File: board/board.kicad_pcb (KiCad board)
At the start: 2 copper layers, 13 parts, among them J1 Conn_01x19, J2 Conn_01x19, J3 Conn_01x02, U1 ESP32-WROVER-E, U2 AOZ1280CI

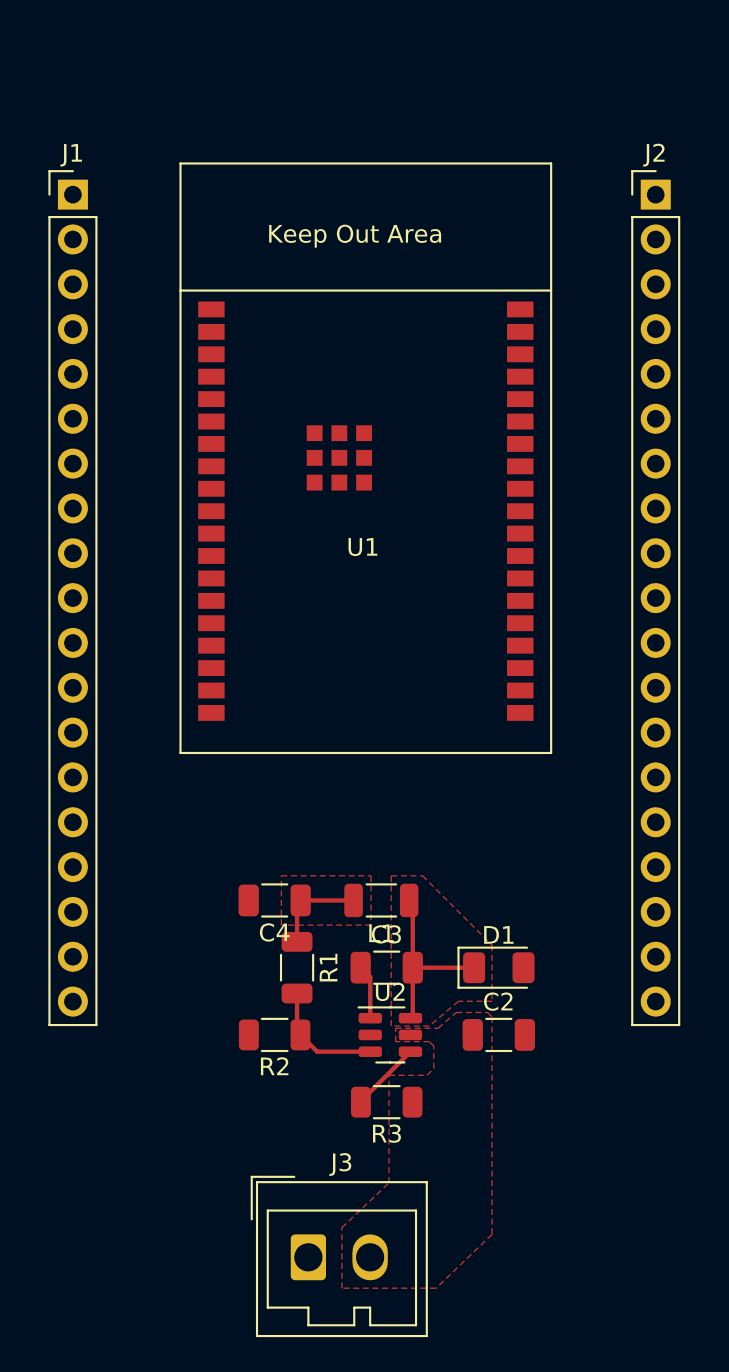
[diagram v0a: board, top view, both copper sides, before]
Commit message: dev
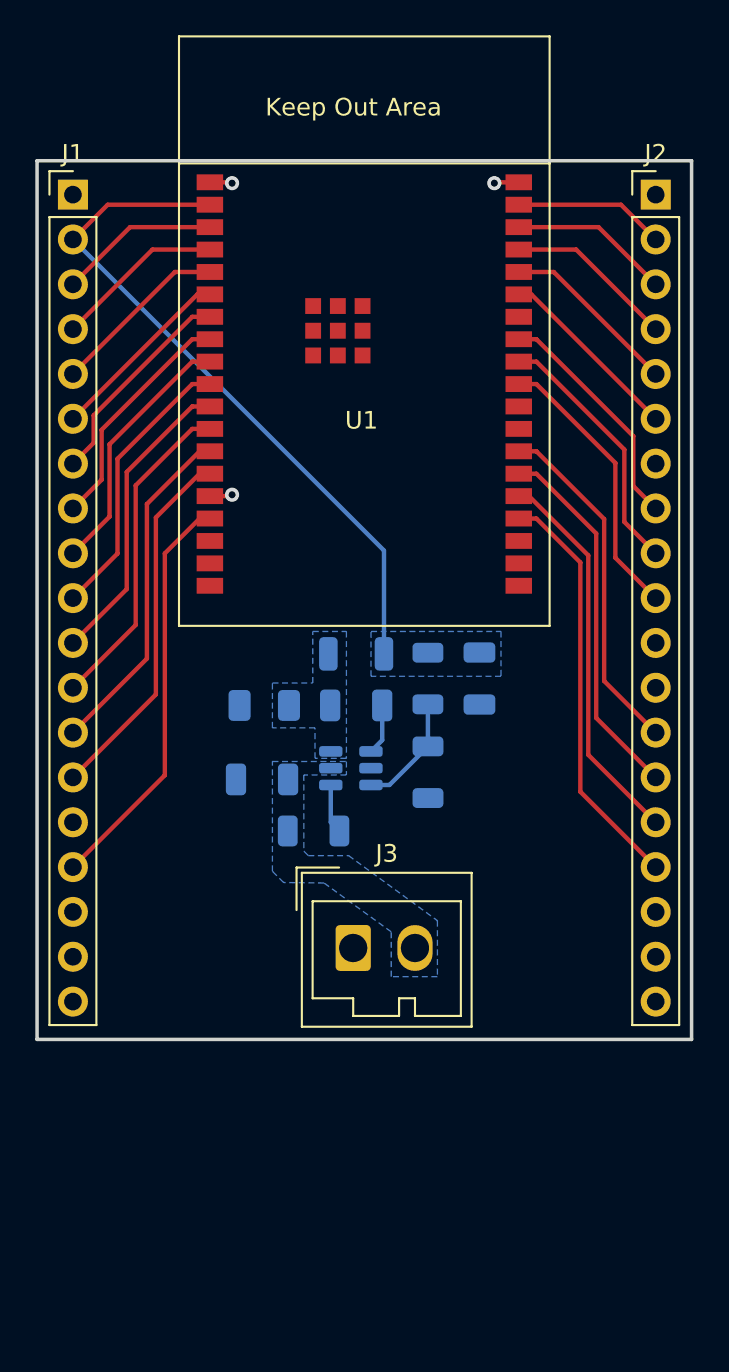
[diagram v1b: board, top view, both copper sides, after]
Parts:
- C2, C3, C4, D1, L1, R1, R2, R3, U2: moved to B.Cu
- moved D1 19.9 mm to (148.0, 84.2), turned to 180 degrees
- moved C2 19.7 mm to (147.9, 88.4), turned to 180 degrees
- moved R1 18.0 mm to (157.3, 82.7)
- moved J3 17.7 mm to (153.0, 97.9)
- moved R2 17.2 mm to (157.3, 88.0), turned to -90 degrees
- moved C4 17.1 mm to (160.2, 82.7), turned to -90 degrees
- moved R3 15.9 mm to (150.8, 91.3), turned to 0 degrees
- moved U2 15.3 mm to (152.9, 87.8), turned to 180 degrees
- moved C3 15.0 mm to (153.2, 84.2), turned to 180 degrees
- moved L1 14.0 mm to (153.2, 81.3), turned to 0 degrees
- moved U1 7.20 mm to (153.7, 66.0)
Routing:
- net 3.3: track 5.43 -> 39.4 mm
- net Net-(J2-Pin_16): track 0.00 -> 23.5 mm
- net Net-(J1-Pin_16): track 0.00 -> 23.3 mm
- net Net-(J2-Pin_15): track 0.00 -> 22.0 mm
- net Net-(J2-Pin_14): track 0.00 -> 21.0 mm
- net Net-(J1-Pin_14): track 0.00 -> 20.8 mm
- net Net-(J2-Pin_13): track 0.00 -> 19.7 mm
- net Net-(J1-Pin_13): track 0.00 -> 19.5 mm
- net Net-(J1-Pin_12): track 0.00 -> 18.5 mm
- net Net-(J1-Pin_11): track 0.00 -> 17.2 mm
- net Net-(J2-Pin_10): track 0.00 -> 15.9 mm
- net Net-(J1-Pin_10): track 0.00 -> 15.9 mm
- net Net-(J2-Pin_9): track 0.00 -> 14.7 mm
- net Net-(J1-Pin_9): track 0.00 -> 14.7 mm
- net Net-(J2-Pin_8): track 0.00 -> 13.4 mm
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- added copper zone on B.Cu, net /VIN
- added copper zone on B.Cu, net /VOUT
- added copper zone on B.Cu, net 3.3
- added copper zone on B.Cu, net GND
- removed copper zone on F.Cu, net /VIN
- removed copper zone on F.Cu, net /VOUT
- removed copper zone on F.Cu, net 3.3
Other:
- board outline added: 37.1 x 49.8 mm

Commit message: dev
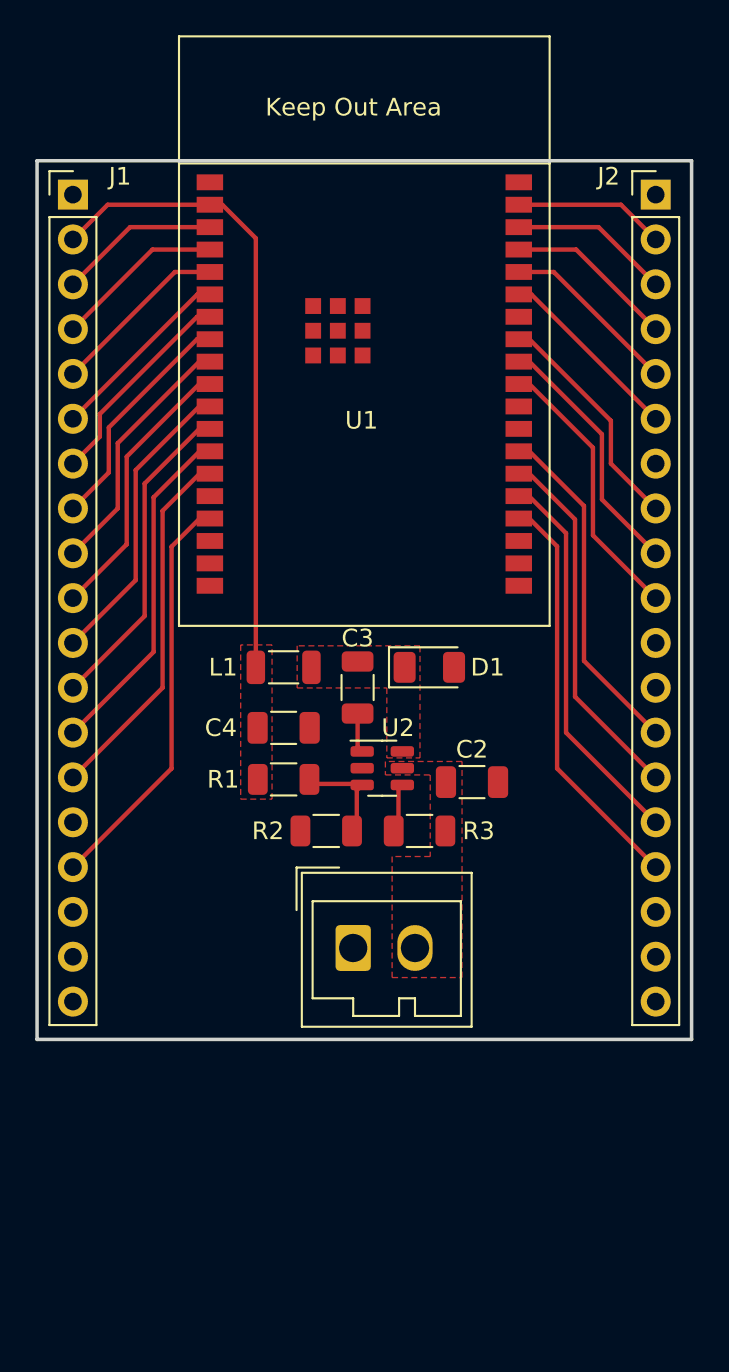
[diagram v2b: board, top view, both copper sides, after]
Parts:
- C2, C3, C4, D1, L1, R1, R2, R3, U2: moved to F.Cu
- moved C2 11.9 mm to (159.8, 88.5), turned to 0 degrees
- moved C4 11.4 mm to (149.1, 85.5), turned to 0 degrees
- moved R1 9.97 mm to (149.1, 88.4), turned to 0 degrees
- moved D1 9.60 mm to (157.4, 82.0), turned to 0 degrees
- moved R2 6.66 mm to (151.5, 91.3), turned to 180 degrees
- moved R3 6.00 mm to (156.8, 91.3), turned to 180 degrees
- moved L1 4.18 mm to (149.1, 82.0), turned to 180 degrees
- moved U2 1.78 mm to (154.7, 87.8), turned to 0 degrees
- moved C3 1.02 mm to (153.3, 83.2), turned to 90 degrees
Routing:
- net GND: track 3.97 -> 0.00 mm, vias 3 -> 0
- net 3.3: track 39.4 -> 36.3 mm
- net Net-(U2-BST): track 2.87 -> 2.25 mm
- net Net-(U2-FB): track 6.52 -> 5.96 mm
- added copper zone on F.Cu, net /VIN
- added copper zone on F.Cu, net /VOUT
- added copper zone on F.Cu, net 3.3
- added copper zone on F.Cu, net GND
- removed copper zone on B.Cu, net /VIN
- removed copper zone on B.Cu, net /VOUT
- removed copper zone on B.Cu, net 3.3

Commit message: dev
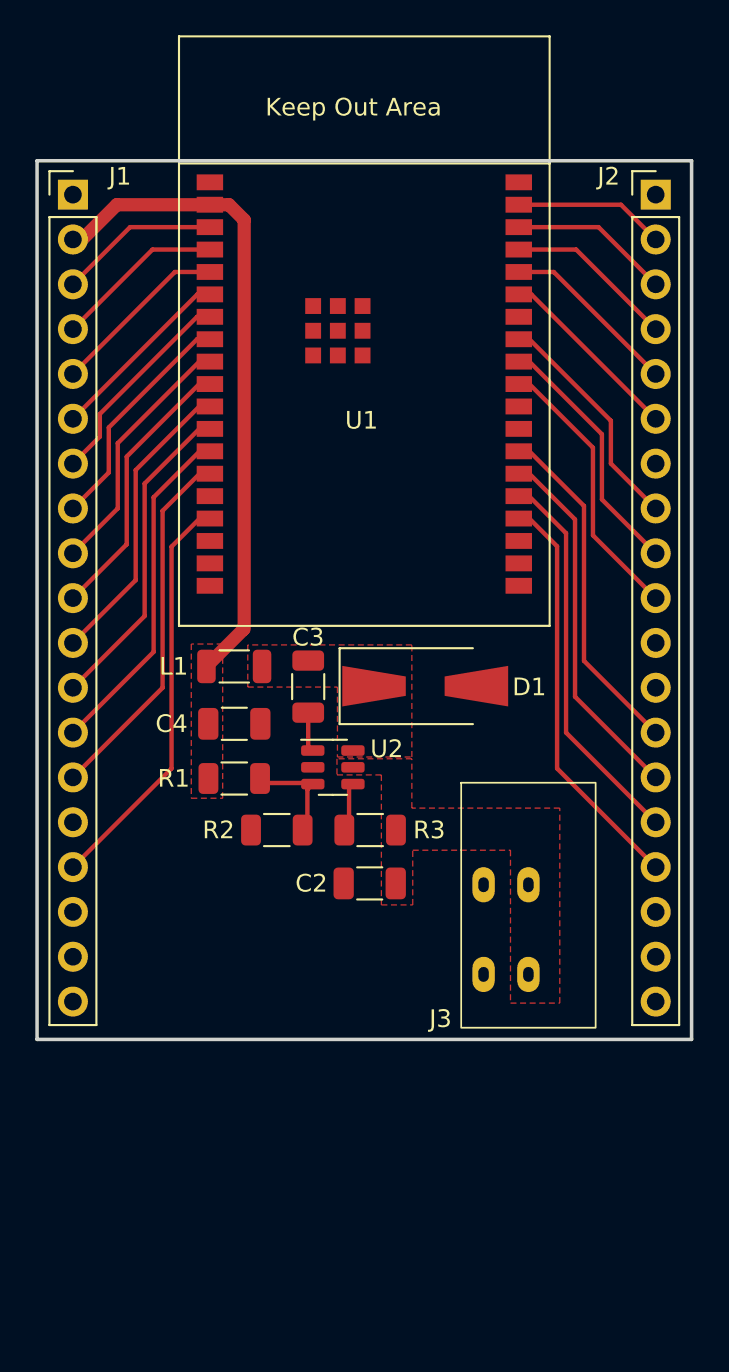
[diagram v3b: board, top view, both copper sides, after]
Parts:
- C2: value C_Small -> 4.7uF
- C3: value C_Small -> 10nF
- C4: value C_Small -> 10uF
- D1: value D_Schottky -> Schottky SMA-SMB; footprint Diode_SMD:D_1206_3216Metric -> Diode_SMD:D_SMA-SMB_Universal_Handsoldering
- J3: value Conn_01x02 -> 3.3-26V; footprint Connector_Wago:Wago_734-132_1x02_P3.50mm_Vertical -> Custom_Connector:Ninigi AC141R-02P-2.54
- L1: value L -> 2.2uH
- R1: value R_Small -> 49.9kΩ
- R2: value R_Small -> 15.8kΩ
- U1: footprint RF_Module_Custom:ESP32-WROVER-IE -> Custom_RF_Module:ESP32-WROVER-IE
- moved C2 8.16 mm to (154.0, 94.3), turned to 180 degrees
- moved J3 7.33 mm to (159.2, 102.0)
- moved C4 2.80 mm to (146.3, 85.2)
- moved L1 2.80 mm to (146.3, 82.0)
- moved R1 2.80 mm to (146.3, 88.3)
- moved C3 2.80 mm to (150.5, 83.1)
- moved R2 2.80 mm to (148.7, 91.3)
- moved R3 2.80 mm to (154.0, 91.3)
- moved U2 2.80 mm to (151.9, 87.7)
- moved D1 1.09 mm to (157.1, 83.1)
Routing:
- net 3.3: track 36.3 -> 37.0 mm
